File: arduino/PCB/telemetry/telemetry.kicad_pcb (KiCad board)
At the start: 2 copper layers, 7 parts, among them J1 Boton Enter, J3 Boton Next, U1 MEGA_PRO_EMBED_CH340G_{slash}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, U2 NEO-M8N

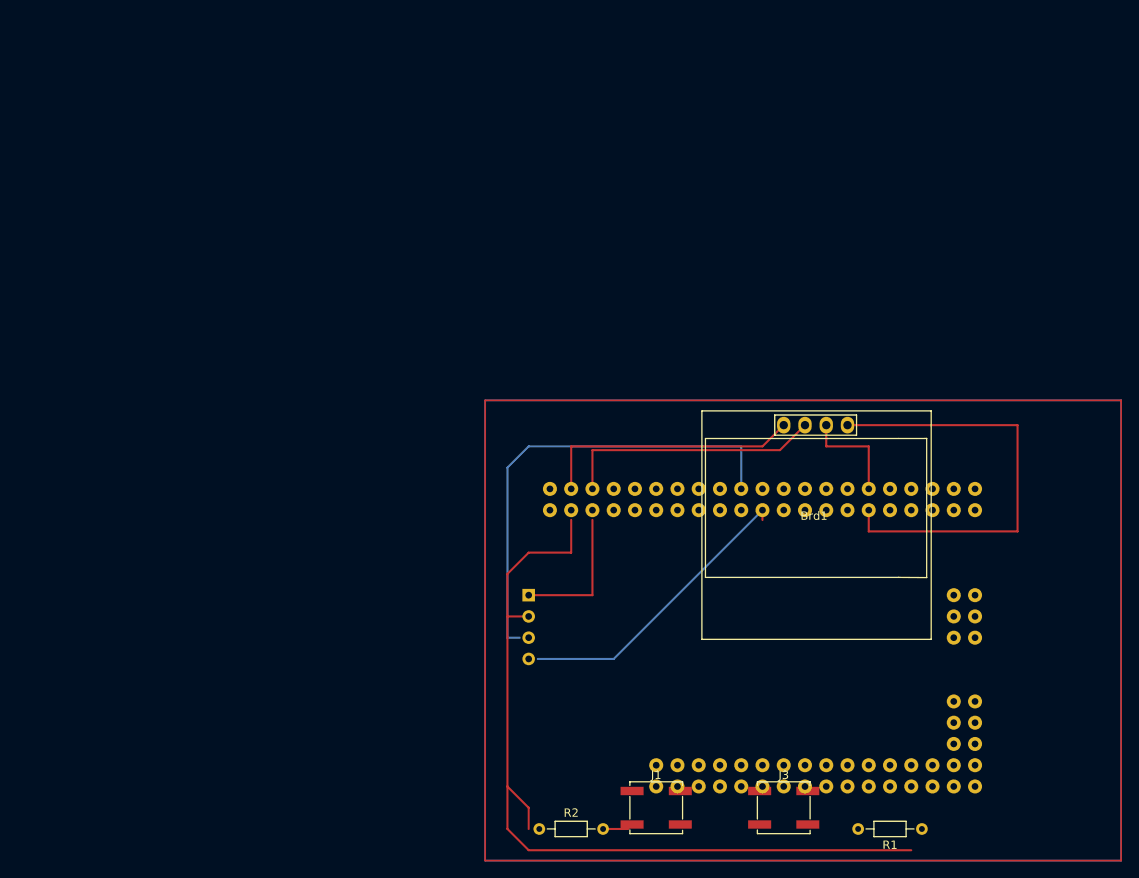
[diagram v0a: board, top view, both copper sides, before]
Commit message: Linear Sensor
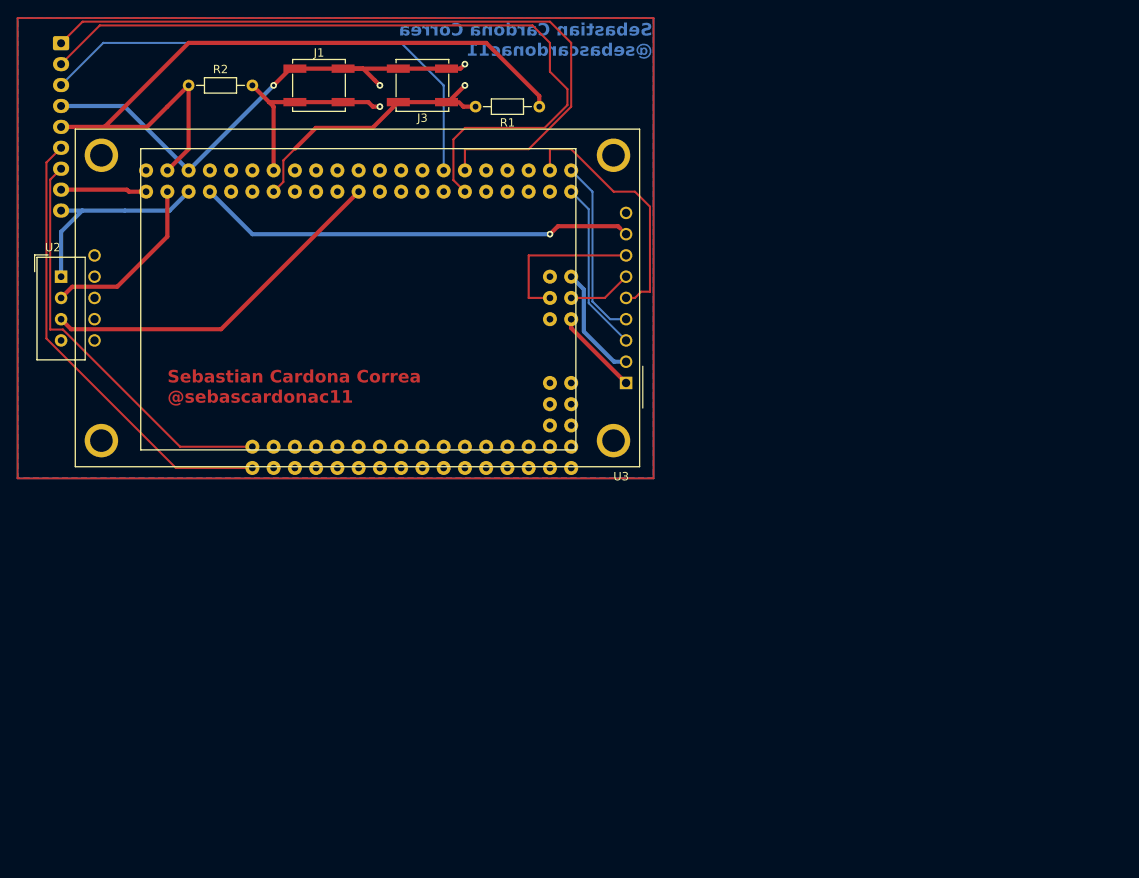
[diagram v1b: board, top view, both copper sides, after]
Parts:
- removed Brd1: SSD1306, SSD1306:128x64OLED
- added J4: DE9_Plug, Connector_JST:JST_EH_S9B-EH_1x09_P2.50mm_Horizontal, B.Cu at (20.3, 15.3)
- added U3: CR2013-MI2120, Display:CR2013-MI2120, F.Cu at (87.8, 55.9)
- U2: moved to F.Cu
- moved R2 98.2 mm to (35.6, 20.4)
- moved R1 97.7 mm to (77.5, 22.9)
- moved J3 96.5 mm to (63.5, 20.4), turned to 180 degrees
- moved J1 95.3 mm to (51.1, 20.4)
- moved U2 67.6 mm to (20.3, 43.2), turned to 0 degrees
- moved U1 61.5 mm to (55.7, 48.3)
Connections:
- U1 pad 3V3_2: Net-(U1-3V3-Pad3V3_1) -> +3.3V
- U1 pad A0: unconnected-(U1-PadA0) -> A0_Suspention
- U1 pad A1: unconnected-(U1-PadA1) -> A1_Suspention
- U1 pad D10: DX_GPS -> TX_GPS
- U1 pad D19: unconnected-(U1-PadD19) -> RPM
- U1 pad D29: unconnected-(U1-PadD29) -> DC
- U1 pad D30: unconnected-(U1-PadD30) -> CS
- U1 pad D31: unconnected-(U1-PadD31) -> RST
- U1 pad MOSI: unconnected-(U1-PadMOSI) -> Net-(U3-MOSI)
- U1 pad SCK: unconnected-(U1-PadSCK) -> Net-(U3-SCK)
- U1 pad VIN_1: Net-(U1-VIN-PadVIN_1) -> (no net)
- U1 pad VIN_2: Net-(U1-VIN-PadVIN_1) -> VIN_2
- U2 pad 1: unconnected-(U2-~{SAFEBOOT}-Pad1) -> +5V
- U2 pad 2: unconnected-(U2-D_SEL-Pad2) -> GND
- U2 pad 3: unconnected-(U2-TIMEPULSE-Pad3) -> TX_GPS
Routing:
- net unconnected-(U2-D_SEL-Pad2): track 101.1 -> 0.00 mm
- net GND: track 31.5 -> 123.5 mm
- net SCL: track 12.7 -> 88.0 mm
- net +5V: track 31.3 -> 96.7 mm, vias 0 -> 3
- net RPM: track 0.00 -> 60.1 mm
- net RX_GPS: track 55.9 -> 0.00 mm
- net A0_Suspention: track 0.00 -> 54.5 mm
- net +3.3V: track 0.00 -> 51.9 mm, vias 0 -> 1
- net A1_Suspention: track 0.00 -> 49.7 mm
- net TX_GPS: track 0.00 -> 42.9 mm
- net SDA: track 53.3 -> 91.6 mm
- net DX_GPS: track 35.4 -> 0.00 mm
- net Net-(J3-Pin_1): track 0.00 -> 33.3 mm, vias 0 -> 1
- net DC: track 0.00 -> 30.7 mm
- net RST: track 0.00 -> 21.6 mm
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- added copper zone on B.Cu, net (none)
- added copper zone on F.Cu, net (none)
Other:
- board text added: "Sebastian Cardona Correa @sebascardonac11"
